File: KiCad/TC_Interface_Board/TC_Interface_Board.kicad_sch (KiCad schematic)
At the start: 30 parts, among them J1 Conn_01x05, J1_24V1 JST_VH_01x04, J1_CN1 JST_VH_01x03, J2 Conn_01x05, J2_CN1 JST_VH_01x02, J3 Conn_01x05, J3_CN1 JST_VH_01x02, J4 Conn_01x05, J5 Conn_01x05, J6 Conn_01x05, J7 Conn_01x05, J8 Conn_01x05, Q1 DTC143E, Q2 DTC143E, U1 MC34063AP

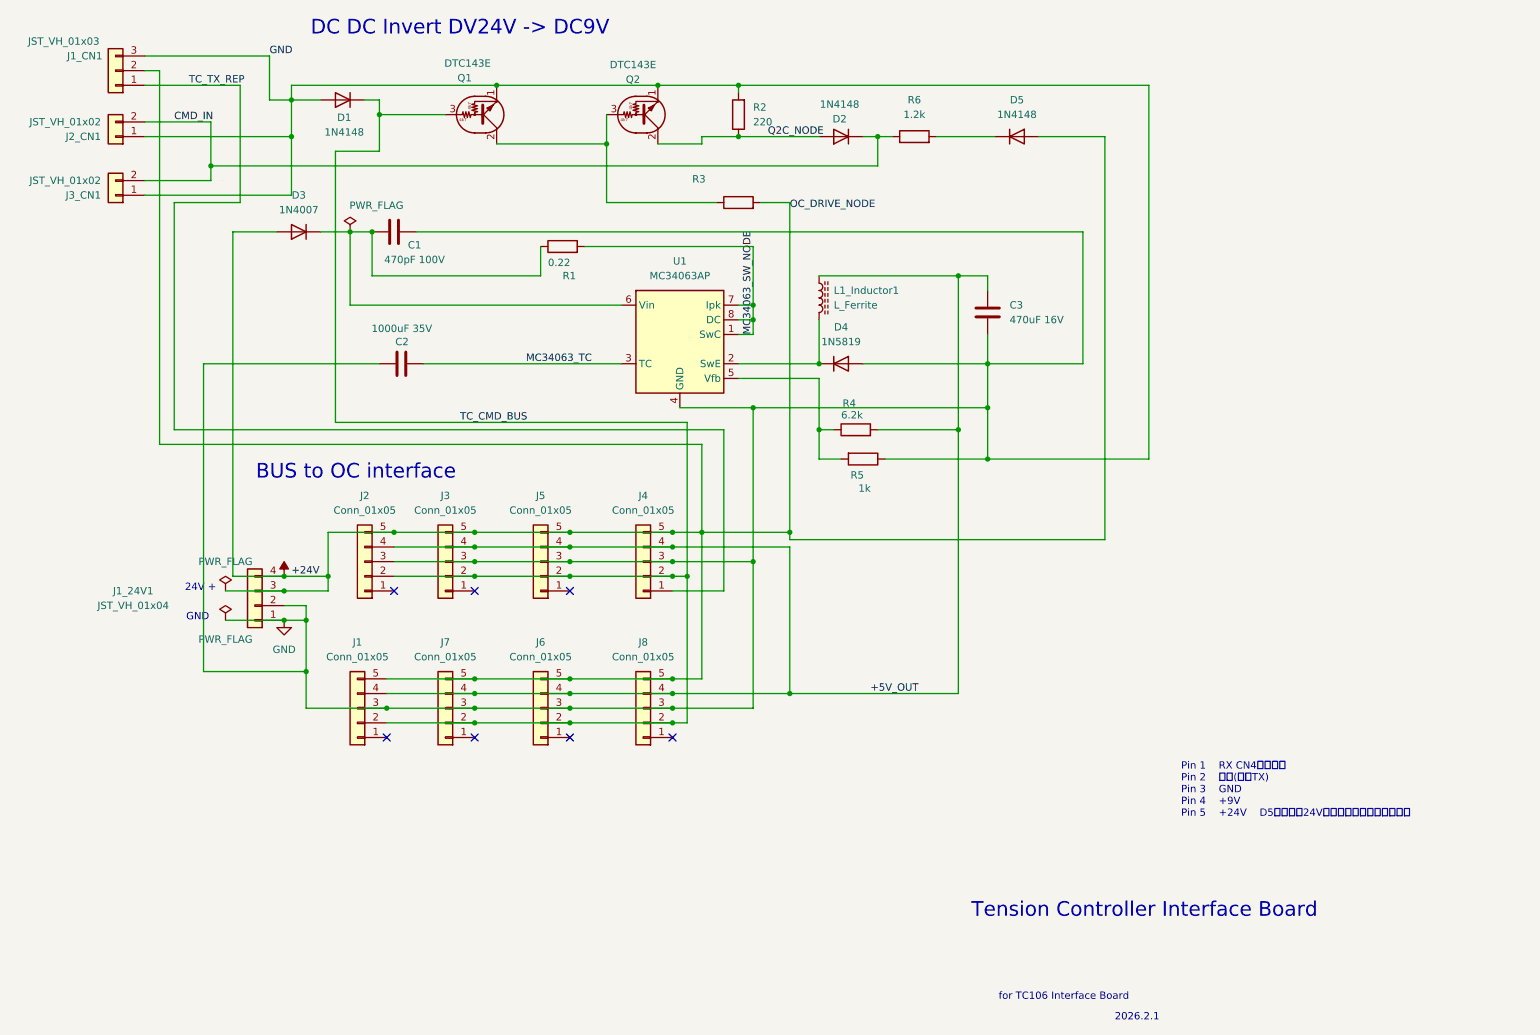
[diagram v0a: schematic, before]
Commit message: UPDATE
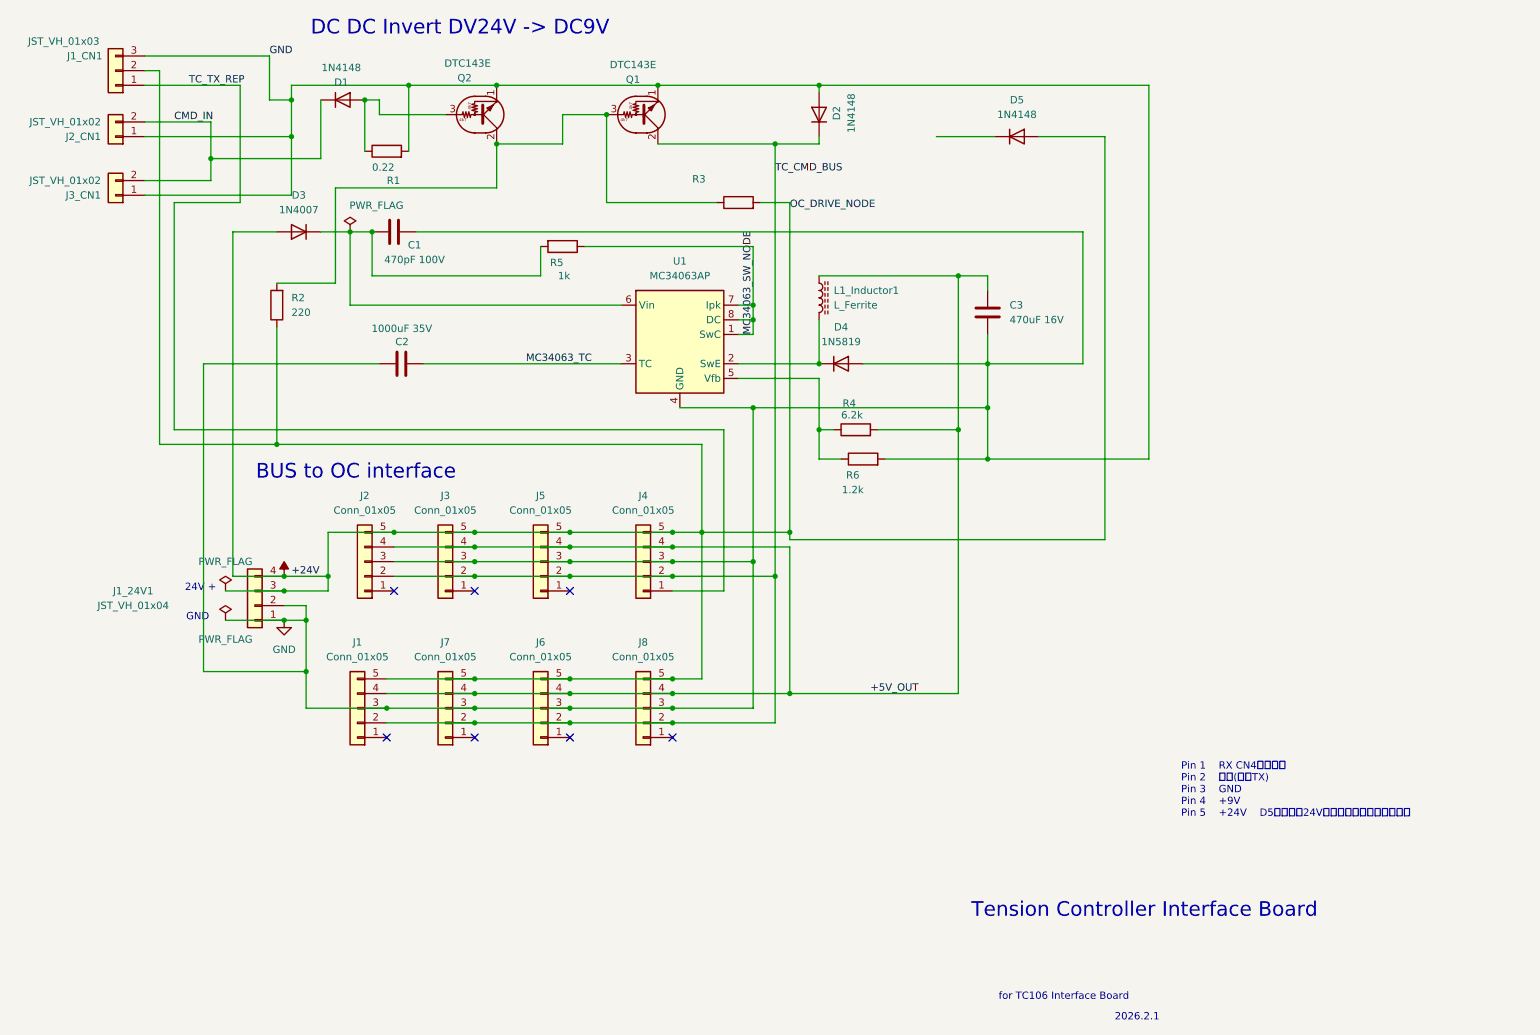
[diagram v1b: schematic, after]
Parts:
- R6: footprint Resistor_THT:R_Axial_DIN0207_L6.3mm_D2.5mm_P15.24mm_Horizontal -> Resistor_THT:R_Axial_DIN0204_L3.6mm_D1.6mm_P7.62mm_Horizontal
- renumbered Q2 to Q1, Q1 to Q2
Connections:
- net +24V: now also R2.1
- net CMD_IN: now also D1.1 (K); no longer D2.1 (K), R6.1
- net GND: now also D2.2 (A), R1.2, R6.2; no longer D1.2 (A), R2.2, R5.1
- net MC34063_SW_NODE: now also R5.1; no longer R1.2
- net TC_CMD_BUS: now also D2.1 (K), Q1.2 (C); no longer D1.1 (K), Q2.3 (B)
- net at D5.1 (K): no longer R6.2
- net at R4.1, U1.5 (Vfb): now also R6.1; no longer R5.2
- net at C1.1, D3.1 (K), U1.6 (Vin): now also R5.2; no longer R1.1
- net at Q1.3 (B), Q2.2 (C), R3.1: now also R2.2
- removed net Q2C_NODE: D2.2 (A), Q1.2 (C), R2.1
- new net: D1.2 (A), Q2.3 (B), R1.1
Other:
- moved on the sheet: D1, D2, R1, R2, R5, R6
